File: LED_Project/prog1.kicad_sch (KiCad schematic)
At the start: 5 parts, among them J1 Conn_01x02, SW1 SW_Push

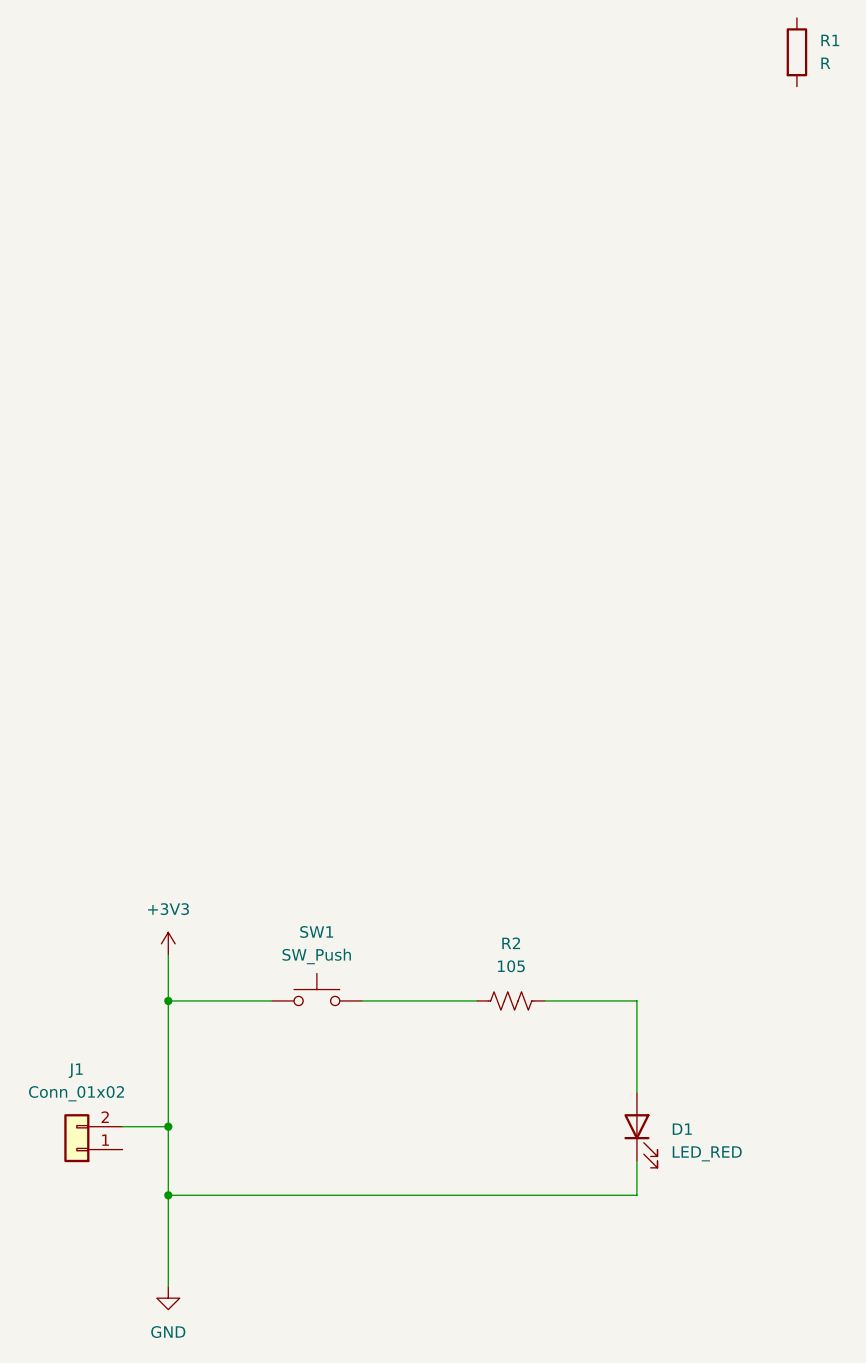
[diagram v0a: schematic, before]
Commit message: completed circuit schematic
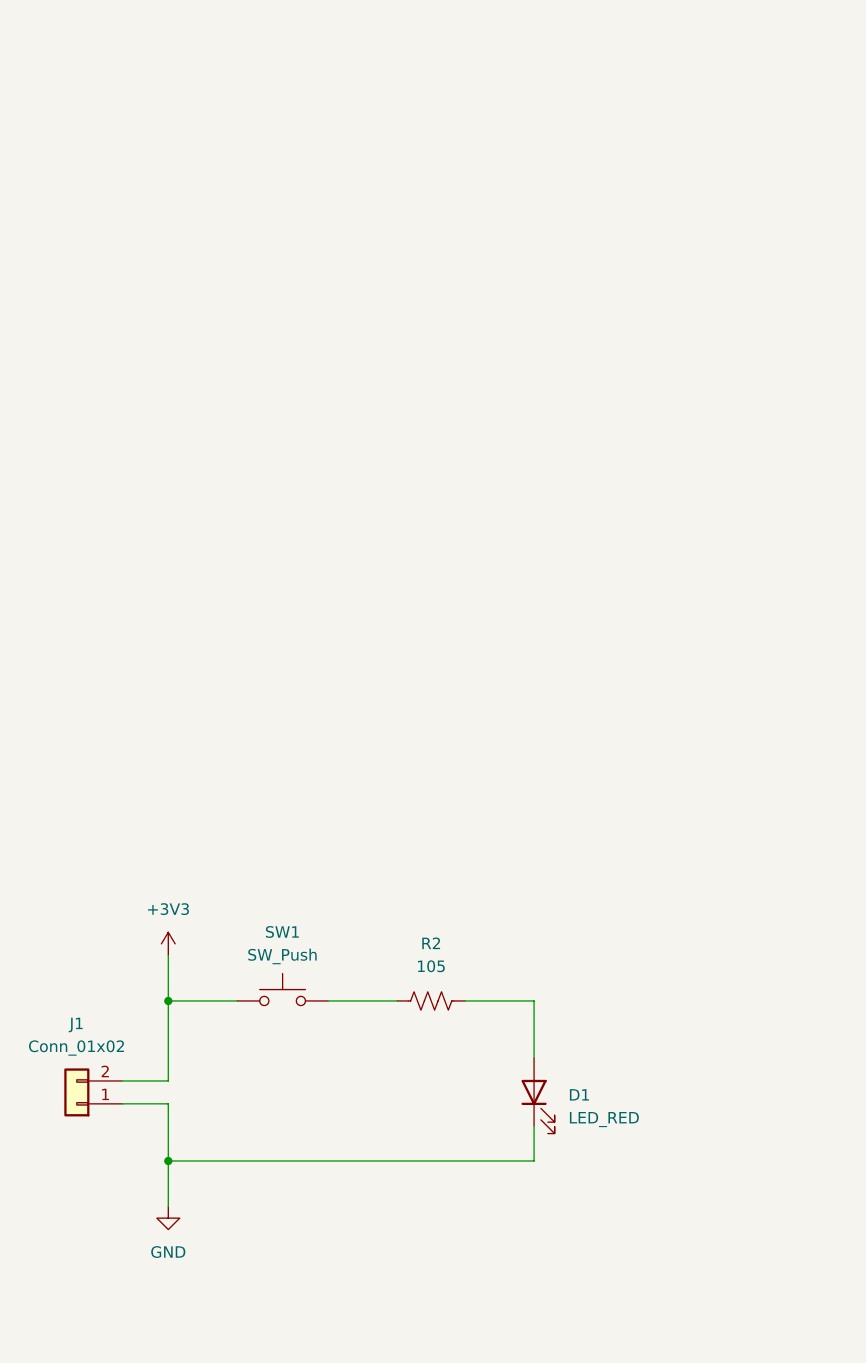
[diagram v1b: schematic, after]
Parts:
- removed R1: R, symbol device:R
- D1: footprint (none) -> layout:LED_0603_Symbol_on_F.SilkS
- J1: footprint (none) -> Connector_Molex:Molex_KK-254_AE-6410-02A_1x02_P2.54mm_Vertical; MPN (none) -> 022272021
- R2: footprint (none) -> Resistor_SMD:R_0603_1608Metric_Pad0.98x0.95mm_HandSolder
- SW1: footprint (none) -> Button_Switch_SMD:SW_DIP_SPSTx01_Slide_6.7x4.1mm_W8.61mm_P2.54mm_LowProfile; MPN (none) -> 1825910-6
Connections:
- net +3V3: no longer D1.1 (K)
- net GND: now reaches J1.1 (Pin_1)
- net GND: now also D1.1 (K)
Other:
- moved on the sheet: D1, J1, R2, SW1
